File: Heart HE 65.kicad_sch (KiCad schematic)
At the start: 61 parts, among them J4 Conn_01x04, J6 Conn_01x04, SW1 SW_Push, U100 STM32F072C8Tx, U19 AP2112K-3.3, U63 AMS1117-3.3, U85 TPS63001, Y1 12Mhz (15p), Y2 8Mhz

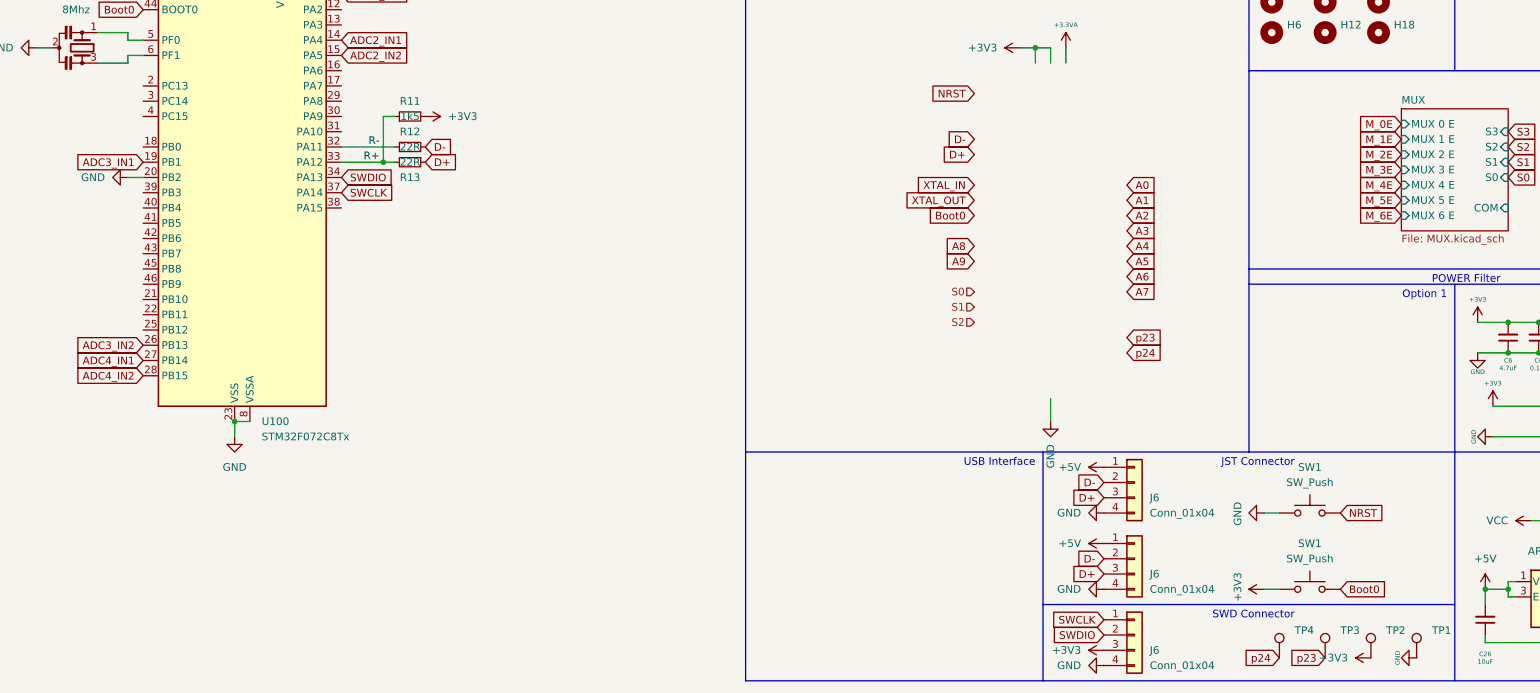
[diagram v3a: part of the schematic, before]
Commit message: Final trace
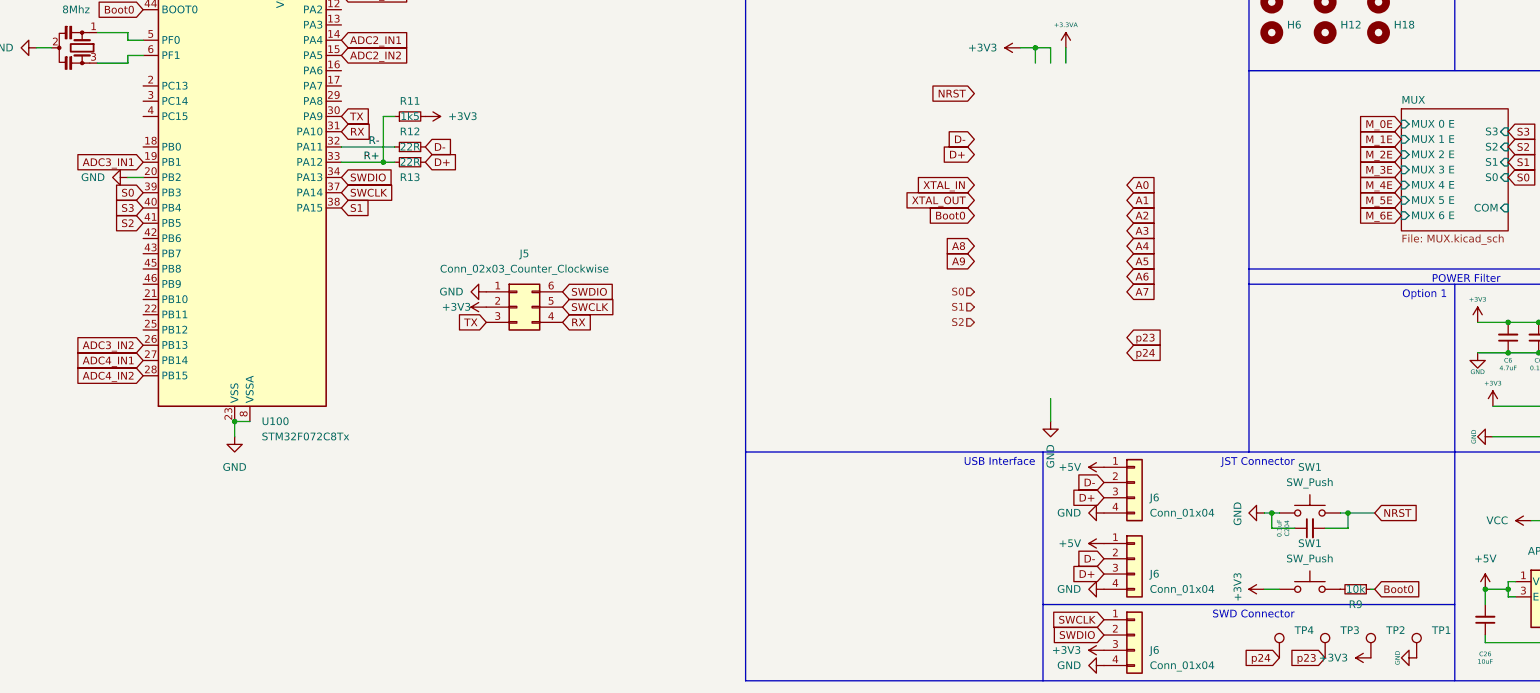
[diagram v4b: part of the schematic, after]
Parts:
- added C204: 0.1uF, Common_Footprint:C_0402, symbol Device:C_Small
- added J5: Conn_02x03_Counter_Clockwise, Connector_PinSocket_2.54mm:PinSocket_2x03_P2.54mm_Vertical, symbol Connector_Generic:Conn_02x03_Counter_Clockwise
- added R9: 10k, Common_Footprint:R_0402, symbol Device:R_Small
- J6: footprint sanproject-keyboard-part:JST-SR-4 -> Common_Footprint:JST-SR-4
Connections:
- net +3.3VA: now also J5.2 (Pin_2)
- net Boot0: now also R9.1; no longer SW1.1
- net GND: now also C204.1, J5.1 (Pin_1)
- net NRST: now also C204.2
- net S0: now also U100.39 (PB3)
- net S1: now also U100.38 (PA15)
- net S2: now also U100.41 (PB5)
- net S3: now also U100.40 (PB4)
- net SWCLK: now also J5.5 (Pin_5)
- net SWDIO: now also J5.6 (Pin_6)
- net TX: now reaches U100.30 (PA9)
- net TX: now also J5.3 (Pin_3)
- net RX: now reaches U100.31 (PA10)
- net RX: now also J5.4 (Pin_4)
- new net: R9.2, SW1.1
